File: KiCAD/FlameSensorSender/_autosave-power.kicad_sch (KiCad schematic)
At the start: 27 parts, among them J5 Conn_01x06_Socket, J6 Conn_01x06_Pin, J7 6 Pin USB-C Type USB Connecto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, Q3 AO3400A, U3 TPS63802DLAR, U4 TPS2116DRL, U5 TPS63802DLAR

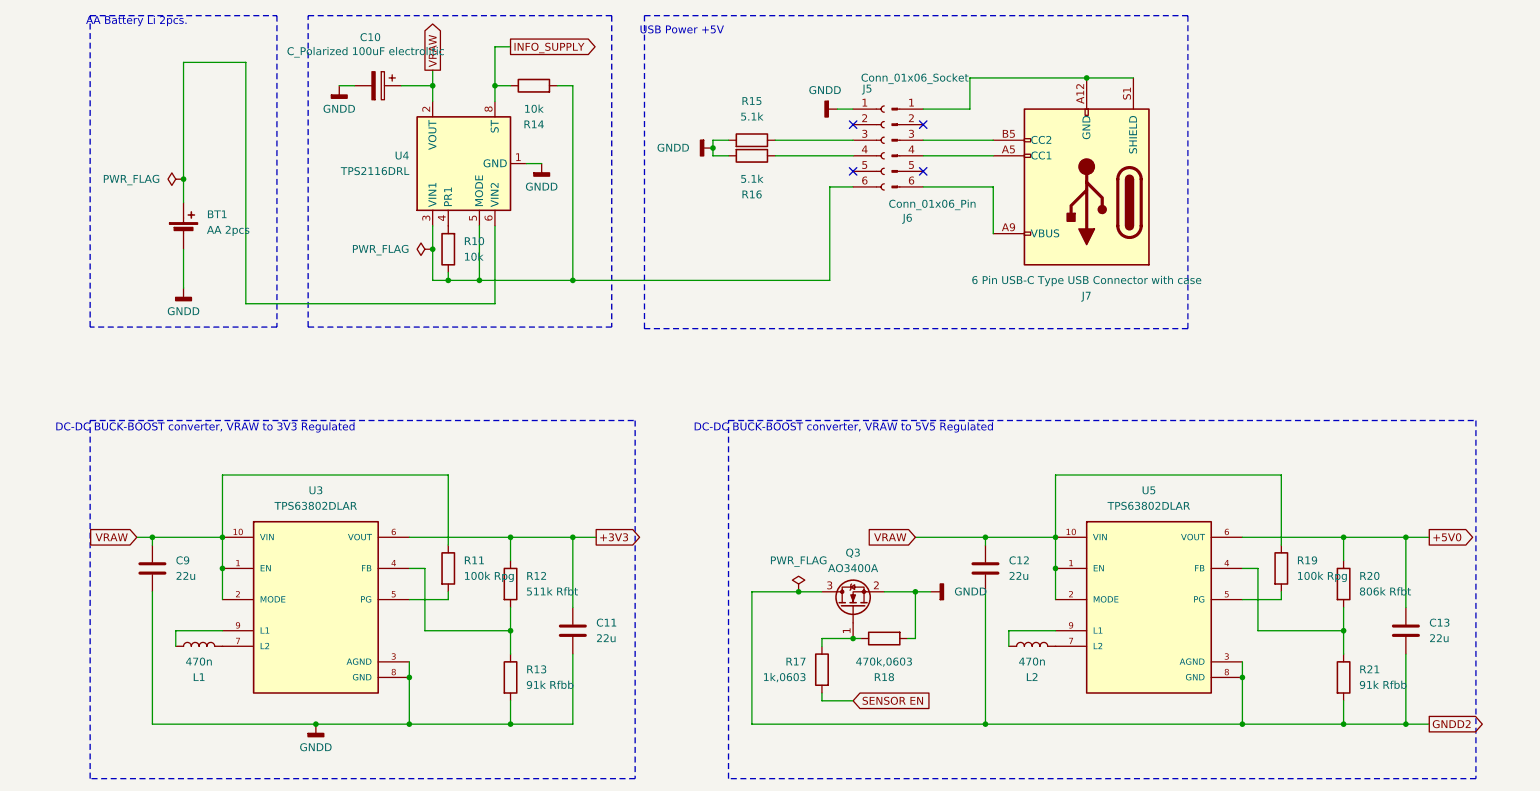
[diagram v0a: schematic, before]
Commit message: dev
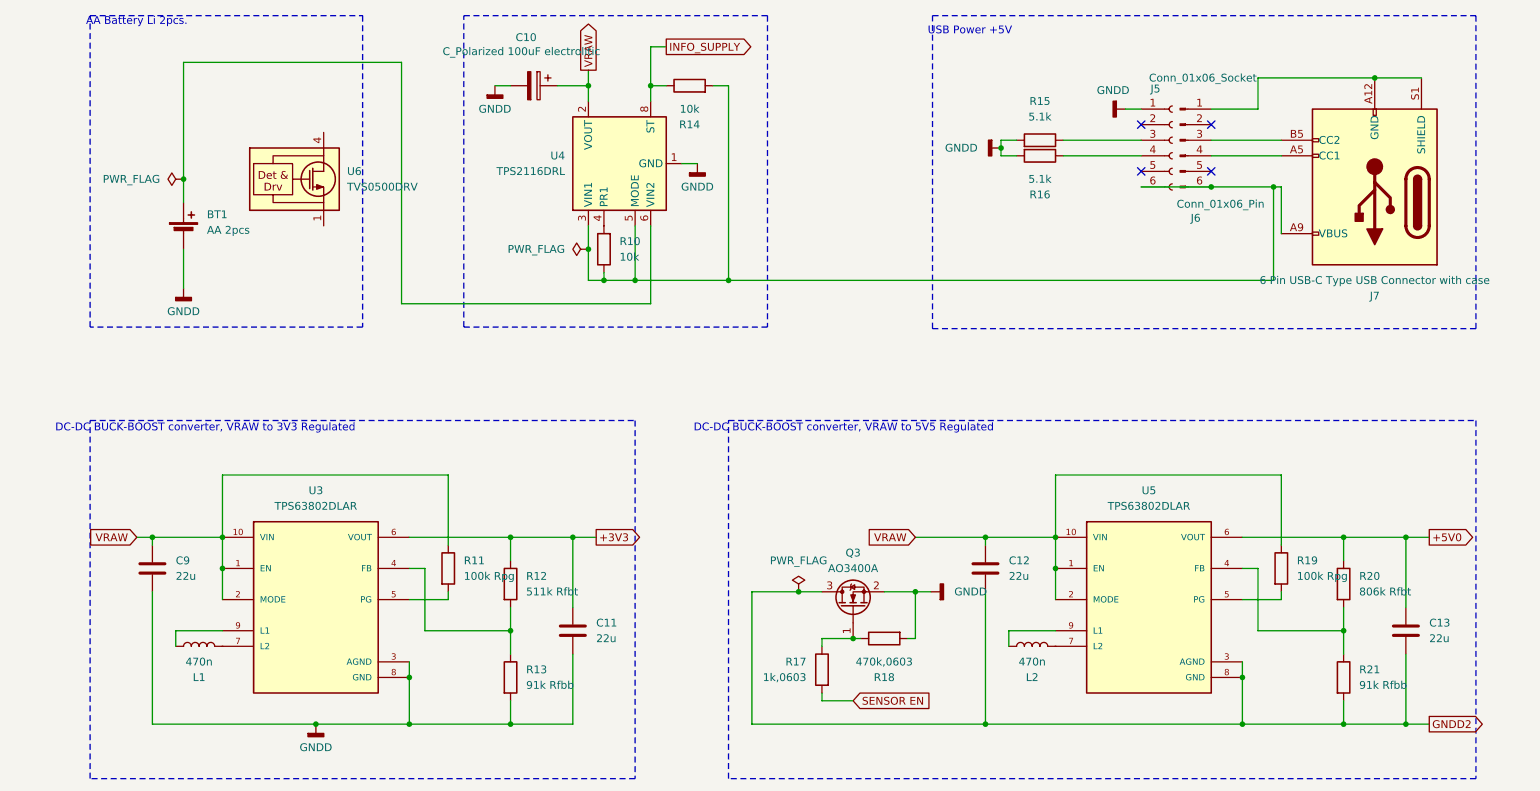
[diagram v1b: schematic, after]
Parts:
- added U6: TVS0500DRV, Package_SON:WSON-6-1EP_2x2mm_P0.65mm_EP1x1.6mm, symbol Power_Protection:TVS0500DRV
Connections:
- net at J5.6 (Pin_6), R10.1, R14.2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: now also J6.6 (Pin_6), J7.A9 (VBUS), J7.B9 (VBUS)
- new net: U6.1 (GND), U6.2 (GND), U6.3 (GND), U6.7 (GND)
- new net: U6.4 (IN), U6.5 (IN), U6.6 (IN)
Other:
- moved on the sheet: C10, J5, J6, J7, R10, R14, R15, R16, U4
